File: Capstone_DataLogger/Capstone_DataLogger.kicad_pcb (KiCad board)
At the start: 2 copper layers, 70 x 130 mm, 27 parts, among them J1 S2B-PH-K-SLFSN, J10 RJ9, J11 Conn_01x04_Socket, J12 S2B-PH-K-SLFSN, J2 S2B-PH-K-SLFSN, J3 S5B-PH-K-S, J4 S2B-PH-K-SLFSN, J5 S2B-PH-K-SLFSN, J6 Conn_01x08_Pin, J7 S4B-PH-K-SLFSN, J8 S4B-PH-K-SLFSN, J9 S4B-PH-K-SLFSN, U2 ESP32-DEVKITC-32D, U3 ATmega328-P, U4 MCP7940M-I/P, U5 IRLZ34NPBF, Y2 32.768k

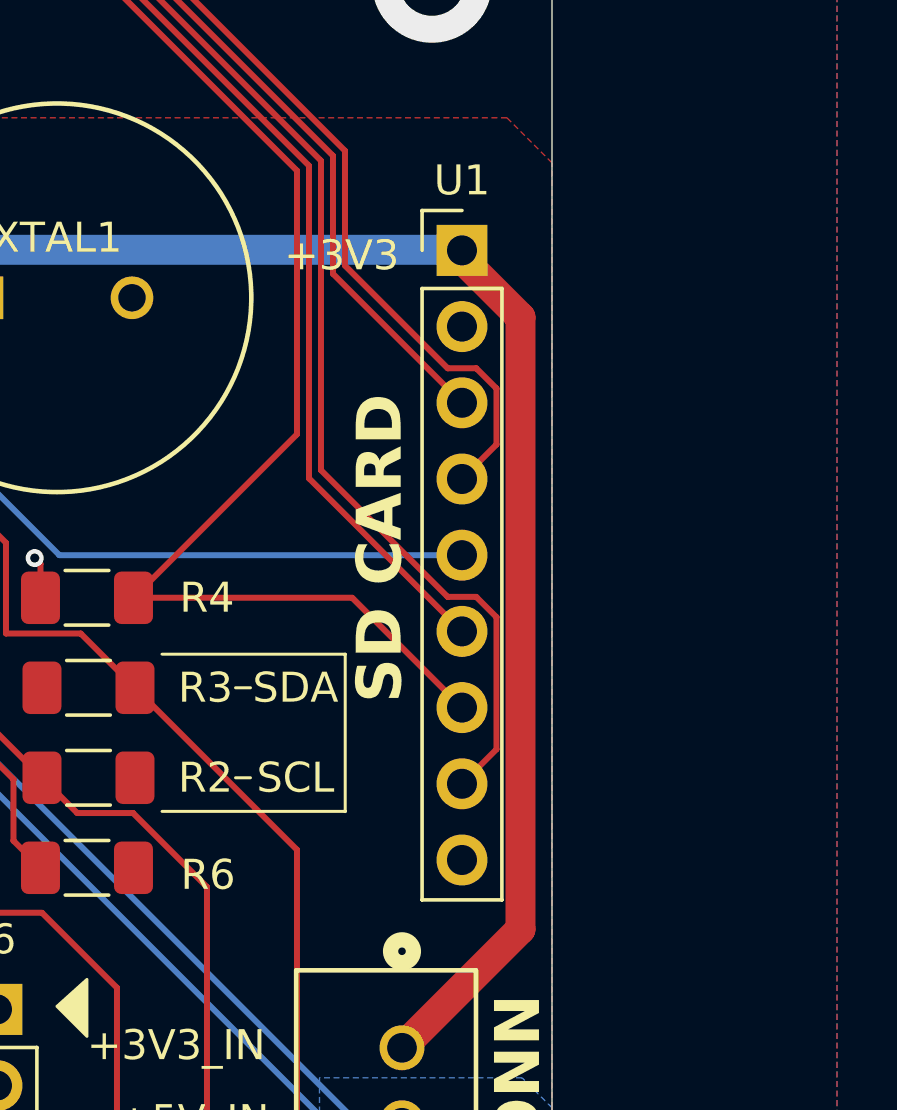
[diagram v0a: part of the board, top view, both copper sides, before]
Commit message: Last revision
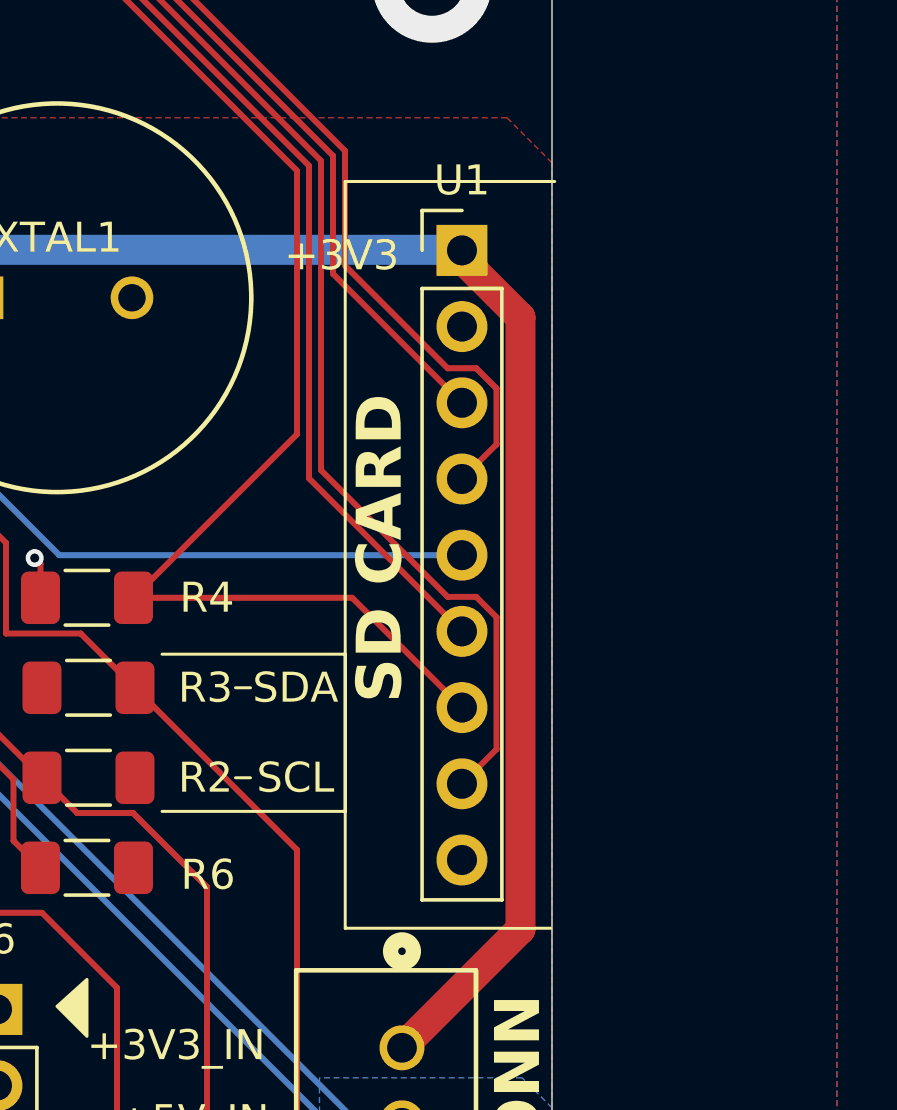
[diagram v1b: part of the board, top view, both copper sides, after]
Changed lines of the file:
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@@
 			(solder_mask_margin 0.102)
 		)
-		(model "C:/Users/mpsch/Downloads/ESP32_DEVKITC_32D/ESP32-DEVKITC-32D.step"
+		(model "${KIPRJMOD}/Capstone.pretty/ESP_Header_Asssembe v1.step"
 			(offset
-				(xyz 0 0 0)
+				(xyz 0 0 9.5)
 			)
 			(scale
@@
 			)
 			(rotate
-				(xyz -90 0 0)
+				(xyz 0 0 0)
 			)
 		)
@@
 	)
 	(gr_line
+		(start 165.608 64.516)
+		(end 172.466 64.516)
+		(stroke
+			(width 0.1)
+			(type default)
+		)
+		(layer "F.SilkS")
+	)
+	(gr_line
+		(start 172.593 39.624)
+		(end 165.608 39.624)
+		(stroke
+			(width 0.1)
+			(type default)
+		)
+		(layer "F.SilkS")
+	)
+	(gr_line
 		(start 159.5 55.38)
 		(end 165.608 55.38)
 		(stroke
 			(width 0.1)
+			(type default)
+		)
+		(layer "F.SilkS")
+	)
+	(gr_line
+		(start 165.608 39.624)
+		(end 165.608 64.516)
+		(stroke
+			(width 0.1)
